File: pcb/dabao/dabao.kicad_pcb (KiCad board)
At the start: 2 copper layers, 134.6 x 90.6 mm, 68 parts, among them J1 Conn_01x05, J2 USB_C_Receptacle_USB2.0_16P, J3 Conn_01x04, J4 MagConn_01x04_Pin, J5 Conn_Battery, J7 Conn_01x04, J8 Display, SW1 SW_RESET, SW2 SW_POWER, U1 nice_nano, U2 MCP23017_SP

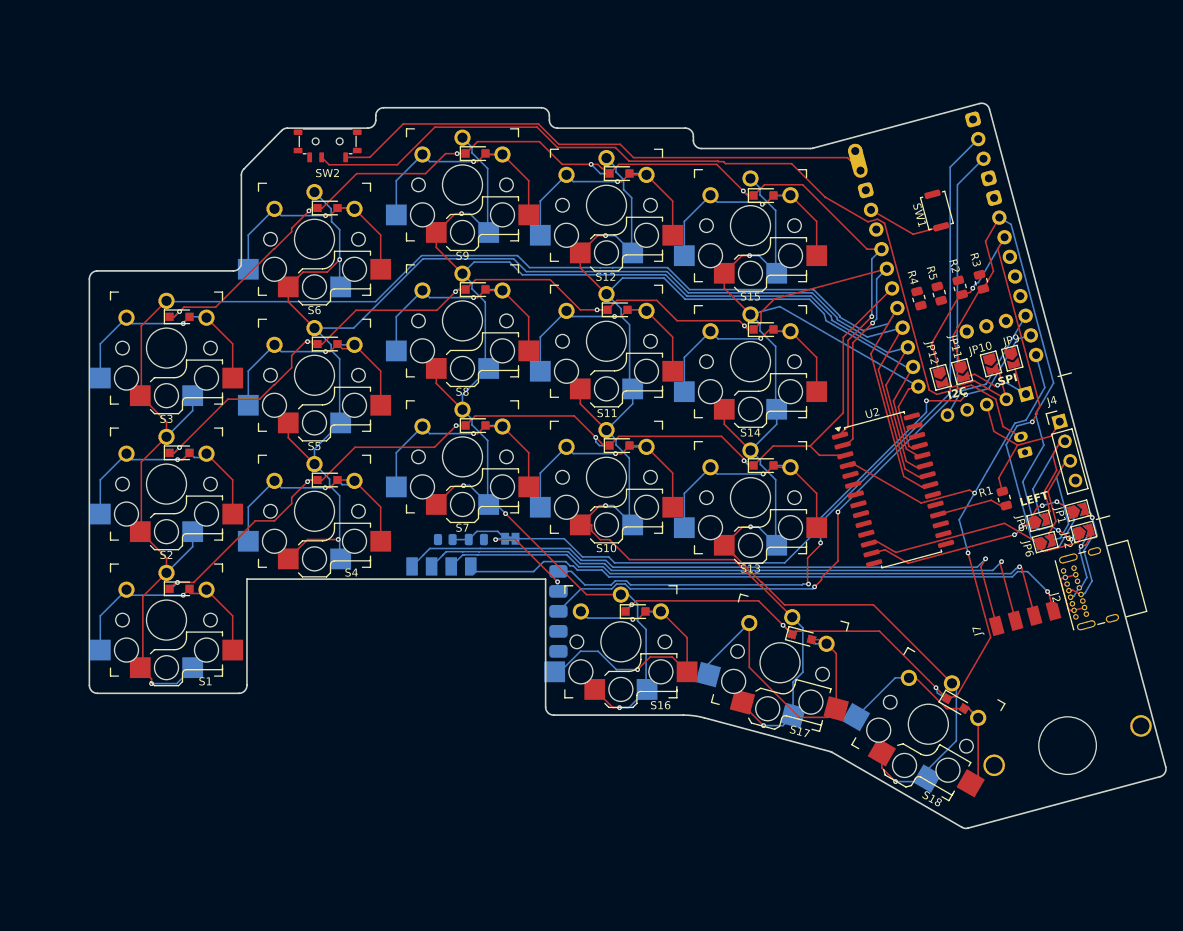
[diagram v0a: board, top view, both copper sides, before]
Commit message: Finish routing
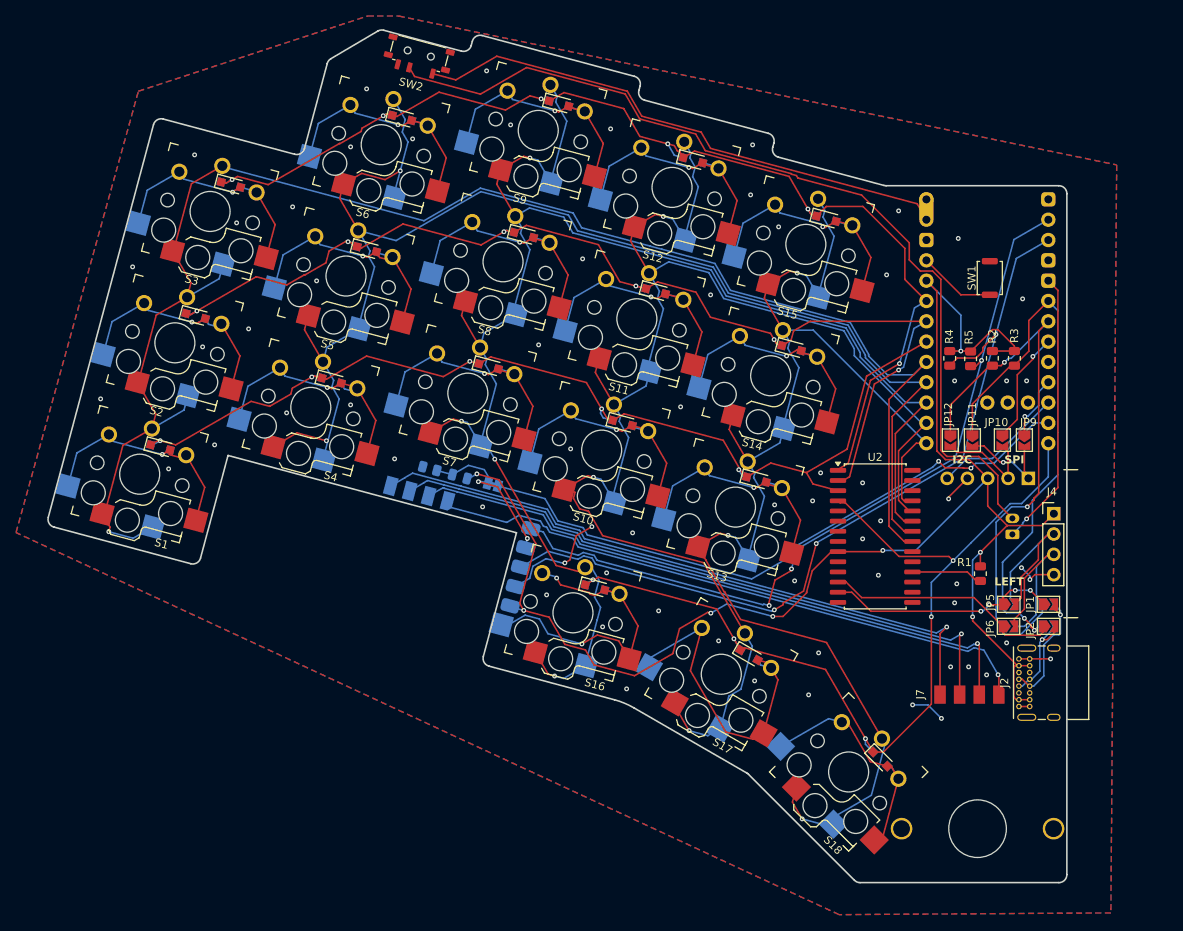
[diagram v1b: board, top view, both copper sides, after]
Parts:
- moved S1 18.5 mm to (98.4, 110.9), turned to -15 degrees
- moved S3 17.9 mm to (107.2, 78.1), turned to -15 degrees
- moved D1 17.8 mm to (101.0, 107.6), turned to -15 degrees
- moved D3 17.7 mm to (109.8, 74.7), turned to -15 degrees
- moved S2 17.7 mm to (102.8, 94.5), turned to -15 degrees
- moved D2 17.2 mm to (105.4, 91.1), turned to -15 degrees
- moved SW2 15.9 mm to (133.3, 58.3), turned to -15 degrees
- moved REF** 15.3 mm to (203.1, 155.2), turned to 90 degrees
- moved D6 14.6 mm to (131.2, 66.4), turned to -15 degrees
- moved S6 14.5 mm to (128.6, 69.7), turned to -15 degrees
- moved J2 13.3 mm to (208.3, 140.0), turned to 90 degrees
- moved S5 13.0 mm to (124.2, 86.1), turned to -15 degrees
- moved S4 13.0 mm to (119.8, 102.6), turned to -15 degrees
- moved D5 12.8 mm to (126.8, 82.8), turned to -15 degrees
- moved JP2 12.6 mm to (212.0, 129.9), turned to 0 degrees
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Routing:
- net VDD: track 27.8 -> 196.4 mm, vias 0 -> 8
- net GND: track 0.00 -> 67.0 mm, vias 0 -> 68
- net /SCK: track 0.00 -> 14.0 mm, vias 0 -> 1
- net /MOSI: track 0.00 -> 7.96 mm, vias 0 -> 1
- net /PS2_CLK: track 96.1 -> 103.7 mm, vias 2 -> 3
- net /row_top: track 139.4 -> 141.3 mm
- net /PS2_Data: track 96.9 -> 98.6 mm, vias 2 -> 3
- net Net-(J1-Pin_2): track 19.8 -> 21.1 mm
- net /TP_reset: track 80.0 -> 78.9 mm
- net /col_middle: track 198.1 -> 198.7 mm
- net Net-(D16-A): track 41.6 -> 41.1 mm
- added copper zone on B.Cu, net GND
- added copper zone on F.Cu, net GND
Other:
- board size 134.6 x 90.6 mm -> 127.4 x 106.6 mm
